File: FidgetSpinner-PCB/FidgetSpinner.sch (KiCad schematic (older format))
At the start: 38 parts, among them J1 DBG_CONN, SW1 SW_POWER, SW2 button, U1 STM32L010K8T6, U2 GP2S60

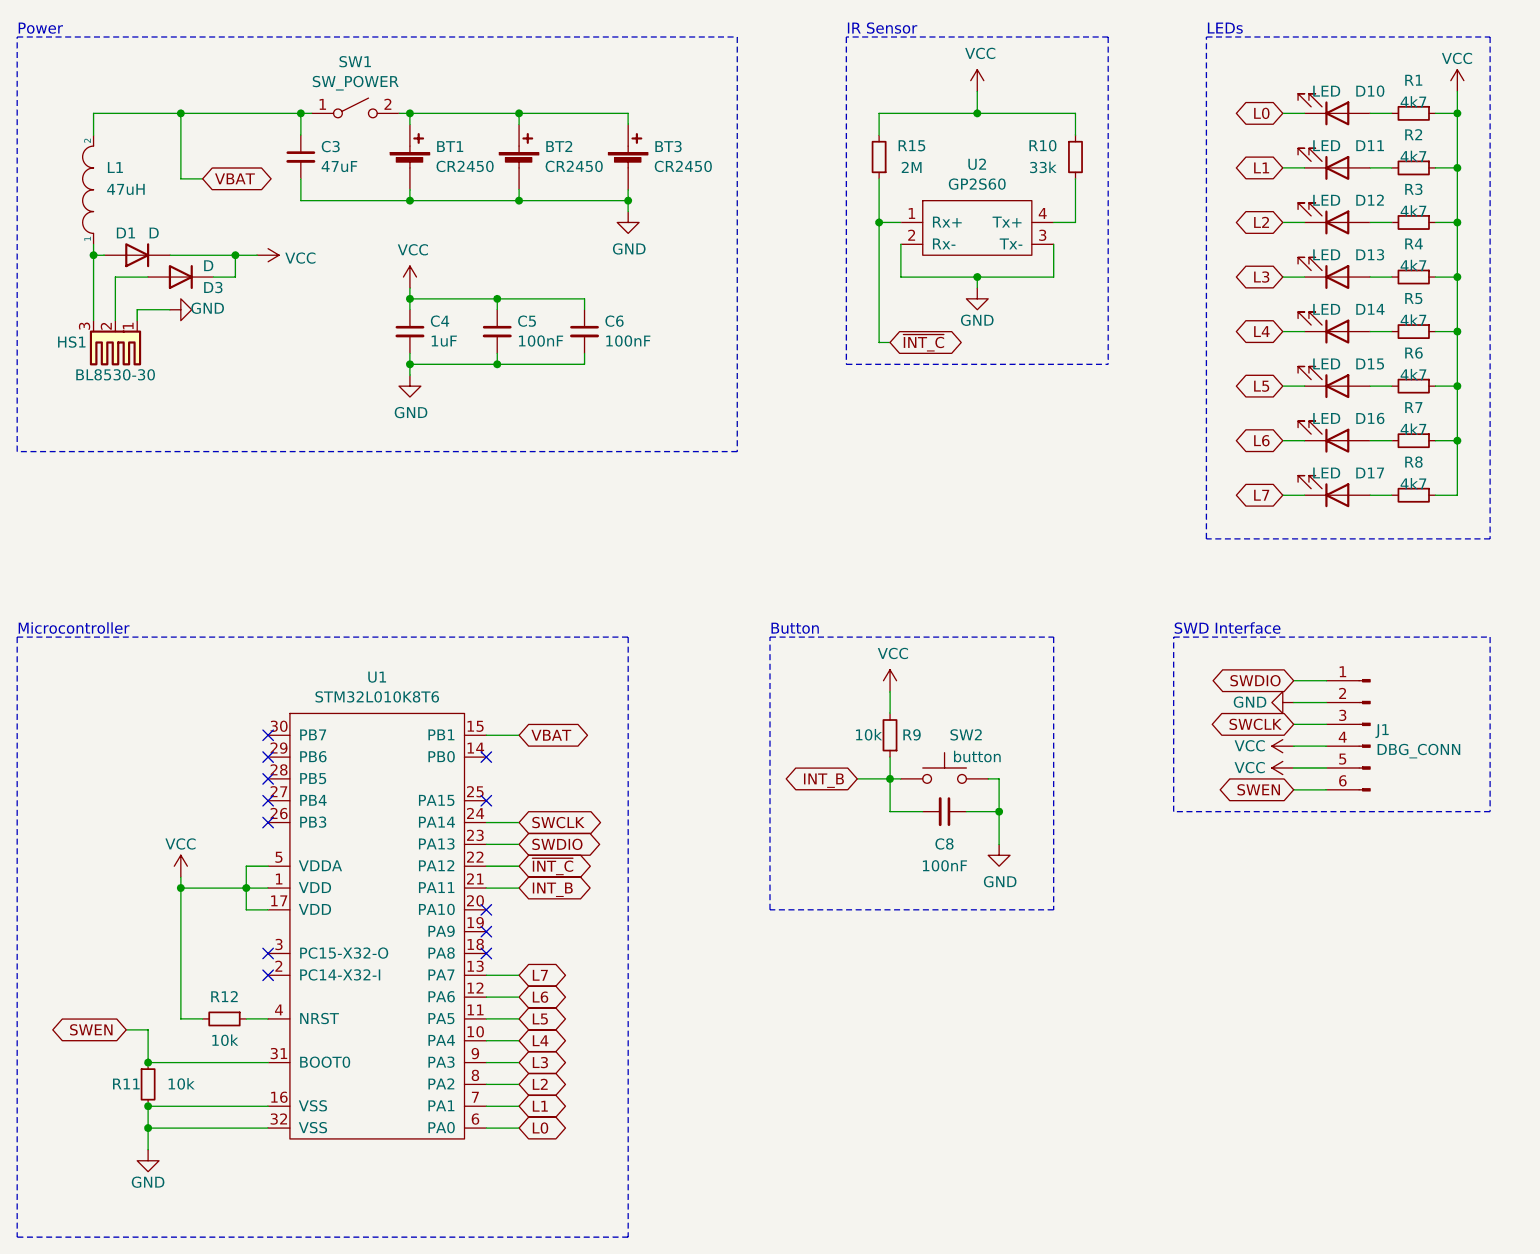
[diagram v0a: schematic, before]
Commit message: backup
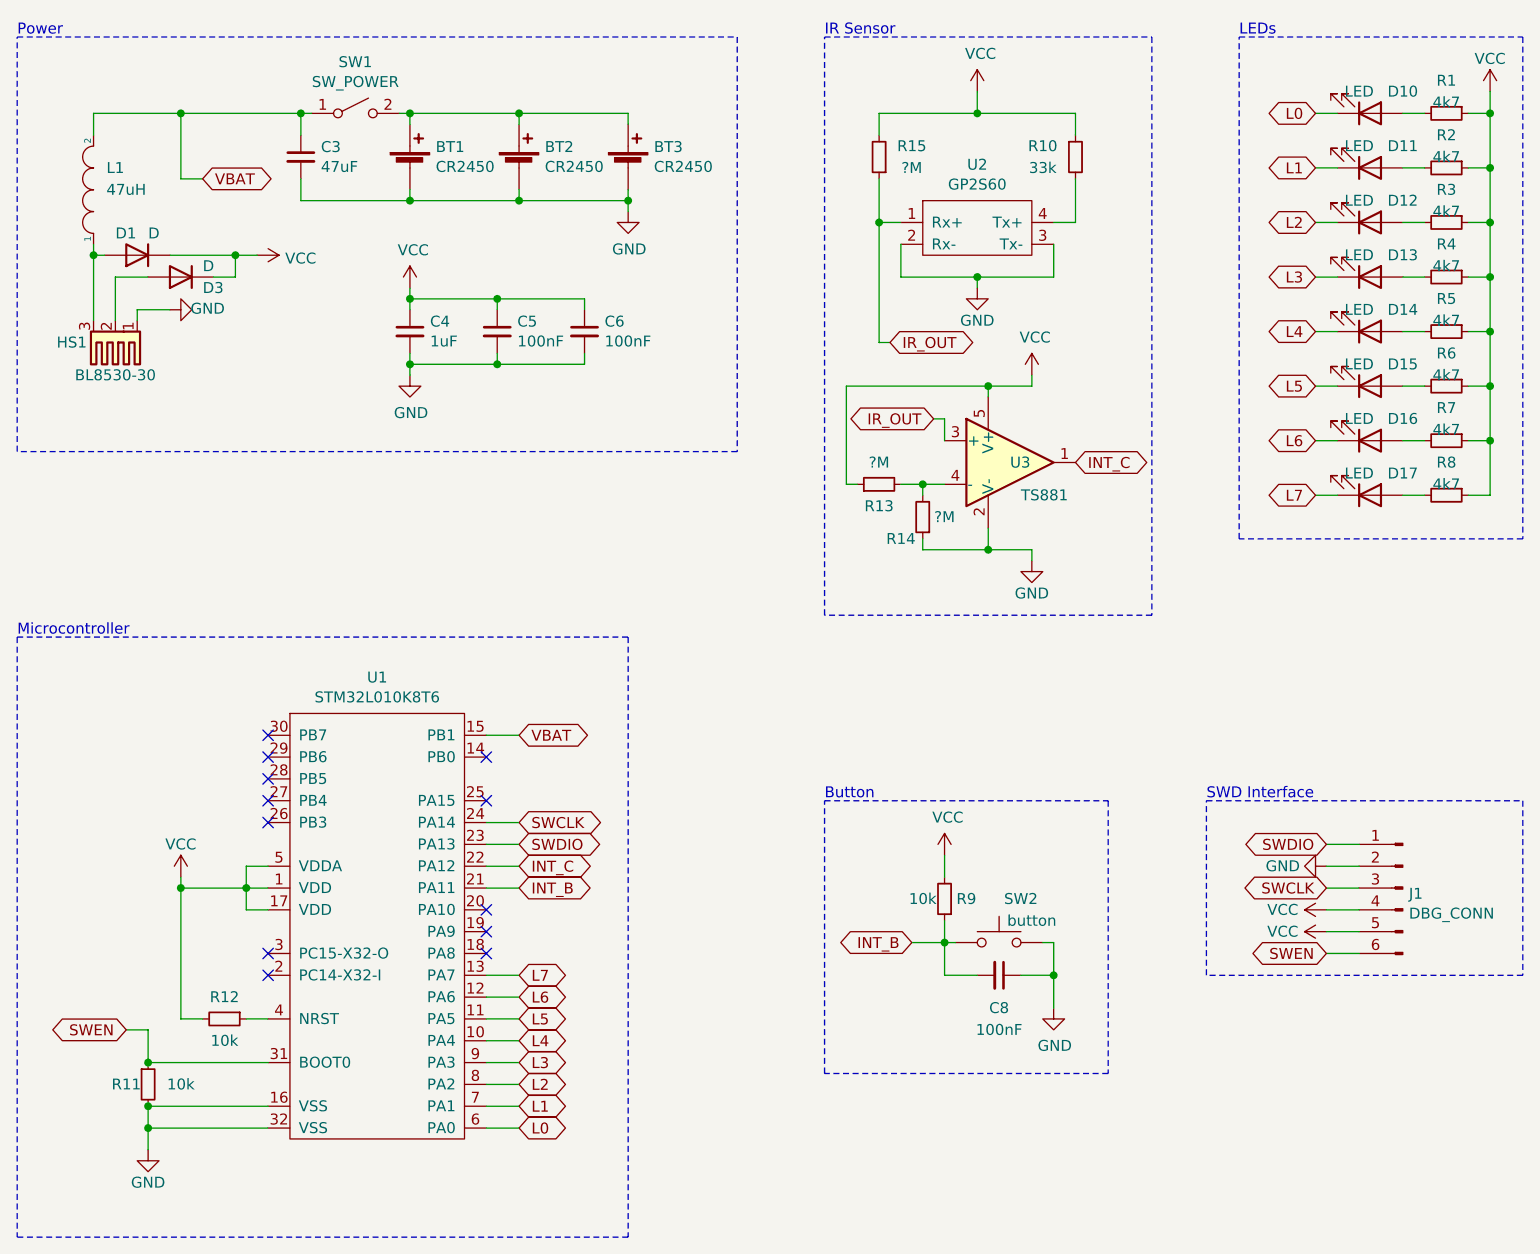
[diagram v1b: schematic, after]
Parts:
- added R13, R14: ?M, Resistor_SMD:R_0805_2012Metric_Pad1.20x1.40mm_HandSolder, symbol Device:R_Small
- added U3: TS881, Package_TO_SOT_SMD:SOT-353_SC-70-5, symbol Amplifier_Operational:TS881xCx
- R15: value 2M -> ?M
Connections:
- net GND: now also R14.1, U3.2 (V-)
- net VCC: now also R13.1, U3.5 (V+)
- net ~INT_C renamed IR_OUT
- net IR_OUT: now also U3.3 (+); no longer U1.22 (PA12)
- new net: R13.2, R14.2, U3.4 (-)
- new net INT_C: U1.22 (PA12), U3.1
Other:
- moved on the sheet: C8, D10, D11, D12, D13, D14, D15, D16, D17, J1, R1, R2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
